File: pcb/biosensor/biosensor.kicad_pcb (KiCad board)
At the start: 2 copper layers, 75 x 65.5 mm, 34 parts, among them J1 Screw_Terminal_01x03, J2 Conn_01x02_Female, P1 USB_C_Plug_USB2.0, SW1 SW_DIP_x01, U1 DW01, U2 TP4056, U3 FS8205A, U4 LM2621

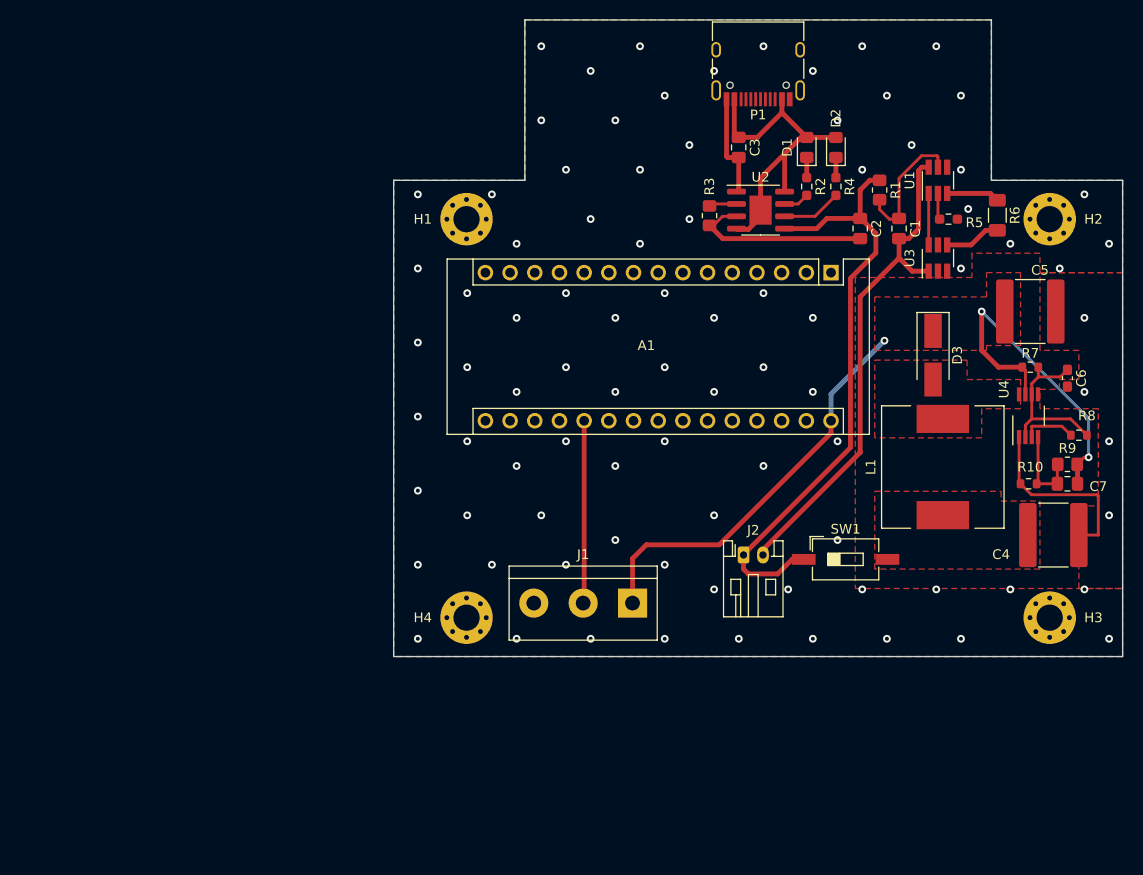
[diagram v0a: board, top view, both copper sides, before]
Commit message: final update?
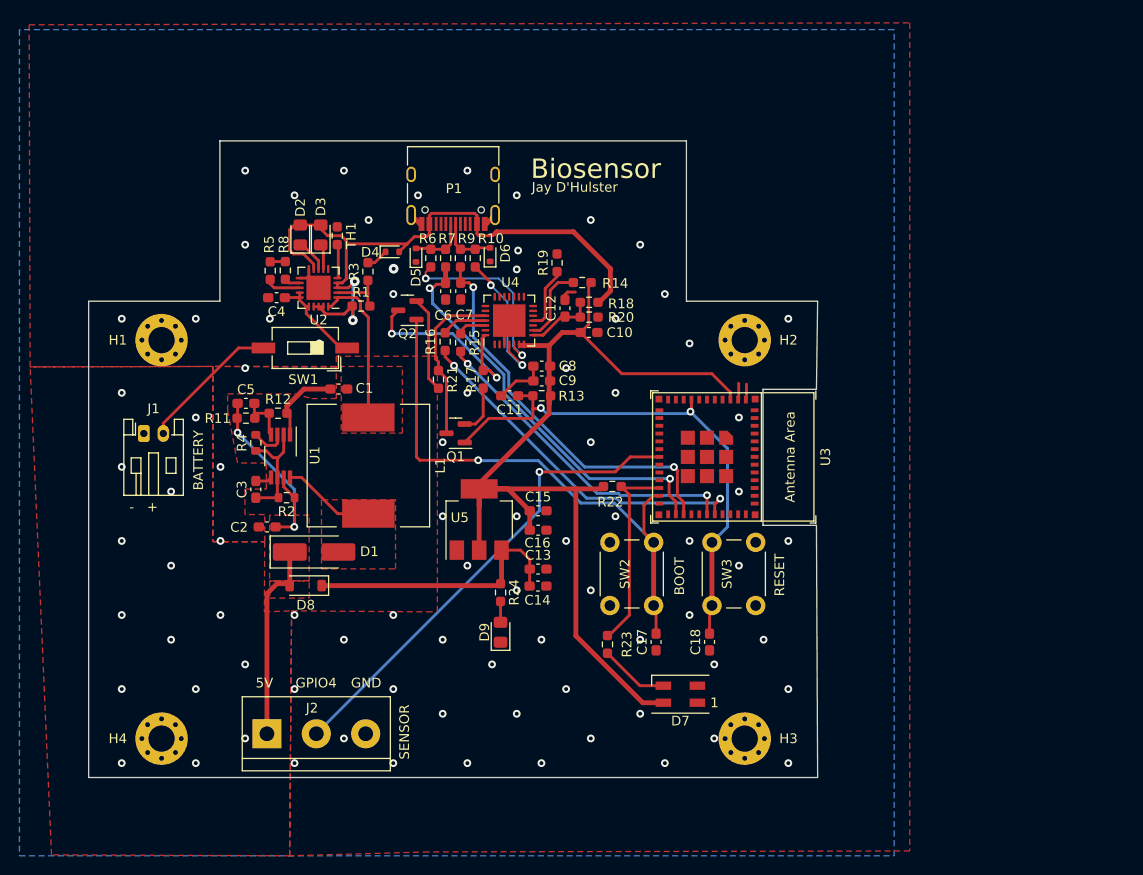
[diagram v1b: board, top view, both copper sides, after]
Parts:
- removed A1: Arduino_Nano_v3.x, Module:Arduino_Nano
- added C10: 10µF/25V/(20%), Capacitor_SMD:C_0603_1608Metric_Pad1.08x0.95mm_HandSolder, F.Cu at (153.6, 86.2)
- added C11: 1µF/16V(10%), Capacitor_SMD:C_0603_1608Metric_Pad1.08x0.95mm_HandSolder, F.Cu at (145.4, 92.7)
- added C12: 1µF/16V(10%), Capacitor_SMD:C_0603_1608Metric_Pad1.08x0.95mm_HandSolder, F.Cu at (151.1, 83.7)
- added C13: 10µF/25V(20%), Capacitor_SMD:C_0603_1608Metric_Pad1.08x0.95mm_HandSolder, F.Cu at (148.4, 110.5)
- added C14: 0.1µF/50V(10%), Capacitor_SMD:C_0603_1608Metric_Pad1.08x0.95mm_HandSolder, F.Cu at (148.3, 112.2)
- added C15: 0.1µF/50V(10%), Capacitor_SMD:C_0603_1608Metric_Pad1.08x0.95mm_HandSolder, F.Cu at (148.4, 104.5)
- added C16: 10µF/25V(20%), Capacitor_SMD:C_0603_1608Metric_Pad1.08x0.95mm_HandSolder, F.Cu at (148.4, 106.5)
- added C17: 0.1µF/50V(10%)(NC), Capacitor_SMD:C_0603_1608Metric_Pad1.08x0.95mm_HandSolder, F.Cu at (160.5, 118.0)
- added C18: 0.1µF/50V(10%)(NC), Capacitor_SMD:C_0603_1608Metric_Pad1.08x0.95mm_HandSolder, F.Cu at (166.0, 118.0)
- added C8: 10µF/25V(20%), Capacitor_SMD:C_0603_1608Metric_Pad1.08x0.95mm_HandSolder, F.Cu at (148.7, 89.6)
- added C9: 0.1µF/50V(10%), Capacitor_SMD:C_0603_1608Metric_Pad1.08x0.95mm_HandSolder, F.Cu at (148.7, 91.1)
- added D4: LESD5D.0CT1G, Diode_SMD:D_SOD-523, F.Cu at (133.4, 77.9)
- added D5: LESD5D.0CT1G, Diode_SMD:D_SOD-523, F.Cu at (135.8, 78.2)
- added D6: LESD5D.0CT1G, Diode_SMD:D_SOD-523, F.Cu at (143.4, 78.2)
- added D7: SK6812MINI, LED_SMD:LED_SK6812MINI_PLCC4_3.5x3.5mm_P1.75mm, F.Cu at (163.0, 123.4)
- added D8: 1N5819HW-7-F, Diode_SMD:D_SOD-123, F.Cu at (124.5, 112.2)
- added D9: RED, LED_SMD:LED_0805_2012Metric_Pad1.15x1.40mm_HandSolder, F.Cu at (144.5, 117.0)
- added Q1: L8050QLT1G, Package_TO_SOT_SMD:SOT-23, F.Cu at (139.9, 96.5)
- added Q2: L8050QLT1G, Package_TO_SOT_SMD:SOT-23, F.Cu at (134.9, 83.9)
- added R11: 150K, Resistor_SMD:R_0603_1608Metric_Pad0.98x0.95mm_HandSolder, F.Cu at (118.3, 95.0)
- added R12: 50K, Resistor_SMD:R_0603_1608Metric_Pad0.98x0.95mm_HandSolder, F.Cu at (121.6, 94.5)
- added R13: 10K(1%), Resistor_SMD:R_0603_1608Metric_Pad0.98x0.95mm_HandSolder, F.Cu at (148.7, 92.7)
- added R14: 1K(1%), Resistor_SMD:R_0603_1608Metric_Pad0.98x0.95mm_HandSolder, F.Cu at (152.9, 81.0)
- added R15: 0(1%), Resistor_SMD:R_0603_1608Metric_Pad0.98x0.95mm_HandSolder, F.Cu at (140.4, 87.2)
- added R16: 0(1%), Resistor_SMD:R_0603_1608Metric_Pad0.98x0.95mm_HandSolder, F.Cu at (138.8, 87.1)
- added R17: 10K(1%), Resistor_SMD:R_0603_1608Metric_Pad0.98x0.95mm_HandSolder, F.Cu at (142.7, 91.0)
- added R18: 22.1K(1%), Resistor_SMD:R_0603_1608Metric_Pad0.98x0.95mm_HandSolder, F.Cu at (153.6, 83.1)
- added R19: 10K(1%)(NC), Resistor_SMD:R_0603_1608Metric_Pad0.98x0.95mm_HandSolder, F.Cu at (150.3, 79.0)
- added R20: 47.5K(1%), Resistor_SMD:R_0603_1608Metric_Pad0.98x0.95mm_HandSolder, F.Cu at (153.6, 84.6)
- added R21: 10K(1%), Resistor_SMD:R_0603_1608Metric_Pad0.98x0.95mm_HandSolder, F.Cu at (138.1, 91.0)
- added R22: 10K(1%), Resistor_SMD:R_0603_1608Metric_Pad0.98x0.95mm_HandSolder, F.Cu at (156.0, 102.0)
- added R23: 0(1%), Resistor_SMD:R_0603_1608Metric_Pad0.98x0.95mm_HandSolder, F.Cu at (155.5, 118.2)
- added R24: 5.1K(1%), Resistor_SMD:R_0603_1608Metric_Pad0.98x0.95mm_HandSolder, F.Cu at (144.5, 112.9)
- added SW2: SW_Push, Button_Switch_THT:SW_PUSH_6mm, F.Cu at (160.2, 107.8)
- added SW3: SW_Push, Button_Switch_THT:SW_PUSH_6mm, F.Cu at (166.2, 114.2)
- added TH1: 16K, Resistor_SMD:R_0603_1608Metric_Pad0.98x0.95mm_HandSolder, F.Cu at (127.7, 76.2)
- added U5: SGM2212-3.3XKC3G/TR, Package_TO_SOT_SMD:SOT-223-3_TabPin2, F.Cu at (142.3, 105.4)
- C1: value 0.1uF -> 22uF; footprint Capacitor_SMD:C_0805_2012Metric_Pad1.18x1.45mm_HandSolder -> Capacitor_SMD:C_0603_1608Metric_Pad1.08x0.95mm_HandSolder
- C2: value 10uF -> 68uF; footprint Capacitor_SMD:C_0805_2012Metric_Pad1.18x1.45mm_HandSolder -> Capacitor_SMD:C_0603_1608Metric_Pad1.08x0.95mm_HandSolder
- C3: value 0.1uF -> 100nF; footprint Capacitor_SMD:C_0805_2012Metric_Pad1.18x1.45mm_HandSolder -> Capacitor_SMD:C_0603_1608Metric_Pad1.08x0.95mm_HandSolder
- C4: value 22uF -> 10µF; footprint Capacitor_SMD:C_2225_5664Metric_Pad1.80x6.60mm_HandSolder -> Capacitor_SMD:C_0603_1608Metric_Pad1.08x0.95mm_HandSolder
- C5: value 68uF -> 39pF; footprint Capacitor_SMD:C_2225_5664Metric_Pad1.80x6.60mm_HandSolder -> Capacitor_SMD:C_0603_1608Metric_Pad1.08x0.95mm_HandSolder
- C6: value 100nF -> 22pF/50V/(5%)(NC)
- C7: value 39pF -> 22pF/50V/(5%)(NC); footprint Capacitor_SMD:C_0805_2012Metric_Pad1.18x1.45mm_HandSolder -> Capacitor_SMD:C_0603_1608Metric_Pad1.08x0.95mm_HandSolder
- D1: value RED -> SS34; footprint LED_SMD:LED_0805_2012Metric_Pad1.15x1.40mm_HandSolder -> Diode_SMD:D_SMA_Handsoldering
- D2: value GREEN -> Opladen
- D3: value SS34 -> Klaar; footprint Diode_SMD:D_SMA_Handsoldering -> LED_SMD:LED_0805_2012Metric_Pad1.15x1.40mm_HandSolder
- J1: value Screw_Terminal_01x03 -> Conn_01x02_Female; footprint TerminalBlock:TerminalBlock_bornier-3_P5.08mm -> Connector_JST:JST_PH_S2B-PH-K_1x02_P2.00mm_Horizontal
- J2: value Conn_01x02_Female -> Screw_Terminal_01x03; footprint Connector_JST:JST_PH_S2B-PH-K_1x02_P2.00mm_Horizontal -> TerminalBlock:TerminalBlock_bornier-3_P5.08mm
- R1: value 100 -> 270K; footprint Resistor_SMD:R_0805_2012Metric_Pad1.20x1.40mm_HandSolder -> Resistor_SMD:R_0603_1608Metric_Pad0.98x0.95mm_HandSolder
- R10: value 50K -> 0(1%); footprint Resistor_SMD:R_0603_1608Metric -> Resistor_SMD:R_0603_1608Metric_Pad0.98x0.95mm_HandSolder
- R2: value 1k -> 500R; footprint Resistor_SMD:R_0603_1608Metric_Pad0.98x0.95mm_HandSolder -> Resistor_SMD:R_0603_1608Metric
- R3: value 10k -> 100K; footprint Resistor_SMD:R_0805_2012Metric_Pad1.20x1.40mm_HandSolder -> Resistor_SMD:R_0603_1608Metric_Pad0.98x0.95mm_HandSolder
- R4: value 1k -> 200K; footprint Resistor_SMD:R_0603_1608Metric_Pad0.98x0.95mm_HandSolder -> Resistor_SMD:R_0603_1608Metric
- R5: value 1k -> 1K
- R6: value 0R -> 0(1%); footprint Resistor_SMD:R_1206_3216Metric_Pad1.30x1.75mm_HandSolder -> Resistor_SMD:R_0603_1608Metric_Pad0.98x0.95mm_HandSolder
- R7: value 500R -> 0(1%)(NC); footprint Resistor_SMD:R_0603_1608Metric -> Resistor_SMD:R_0603_1608Metric_Pad0.98x0.95mm_HandSolder
- R8: value 200K -> 100K; footprint Resistor_SMD:R_0603_1608Metric -> Resistor_SMD:R_0603_1608Metric_Pad0.98x0.95mm_HandSolder
- R9: value 150K -> 0(1%)(NC); footprint Resistor_SMD:R_0805_2012Metric_Pad1.20x1.40mm_HandSolder -> Resistor_SMD:R_0603_1608Metric_Pad0.98x0.95mm_HandSolder
- U1: value DW01 -> LM2621; footprint Package_TO_SOT_SMD:SOT-23-6_Handsoldering -> Package_SO:VSSOP-8_3.0x3.0mm_P0.65mm
- U2: value TP4056 -> MCP73871; footprint Package_SO:SOIC-8-1EP_3.9x4.9mm_P1.27mm_EP2.29x3mm -> Package_DFN_QFN:QFN-20-1EP_4x4mm_P0.5mm_EP2.5x2.5mm
- U3: value FS8205A -> ESP32-C3-MINI-1; footprint Package_TO_SOT_SMD:SOT-23-6_Handsoldering -> Espressif:ESP32-C3-MINI-1
- U4: value LM2621 -> CP2102N-Axx-xQFN28; footprint Package_SO:VSSOP-8_3.0x3.0mm_P0.65mm -> Package_DFN_QFN:QFN-28-1EP_5x5mm_P0.5mm_EP3.35x3.35mm
- moved C4 83.6 mm to (121.5, 82.6), turned to 180 degrees
- moved R8 83.4 mm to (122.4, 79.8), turned to 90 degrees
- moved C5 81.2 mm to (118.3, 93.5)
- moved U1 73.3 mm to (121.9, 98.9), turned to -90 degrees
- moved R5 70.0 mm to (120.8, 79.8), turned to 90 degrees
- moved C2 68.3 mm to (120.5, 106.2), turned to 180 degrees
- moved R9 66.0 mm to (140.4, 78.5), turned to -90 degrees
- moved D1 65.6 mm to (125.3, 108.7), turned to 0 degrees
- moved C7 65.5 mm to (140.4, 81.9), turned to -90 degrees
- moved R4 65.2 mm to (119.3, 97.5), turned to 90 degrees
- moved C6 64.6 mm to (138.8, 81.9)
- moved D3 64.2 mm to (126.0, 76.1), turned to 90 degrees
- moved R2 62.4 mm to (122.5, 103.2), turned to 180 degrees
- moved R10 61.5 mm to (141.9, 78.5), turned to -90 degrees
- moved R7 61.2 mm to (138.8, 78.5), turned to -90 degrees
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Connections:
- C1 pad 1: Net-(C1-Pad1) -> /Load
- C1 pad 2: BAT- -> GND
- C2 pad 1: BAT+ -> +5V
- C3 pad 1: VIN -> Net-(U1-EN)
- C4 pad 1: OUTVCC -> Net-(U2-V_{BAT_SENSE})
- C5 pad 1: /Vout -> +5V
- C5 pad 2: GND -> Net-(U1-FB)
- C6 pad 1: Net-(C6-Pad1) -> /GPIO18
- C7 pad 1: /Vout -> /GPIO19
- C7 pad 2: Net-(C7-Pad2) -> GND
- D1 pad 1: Net-(D1-Pad1) -> +5V
- D1 pad 2: VIN -> /L1
- D2 pad 1: Net-(D2-Pad1) -> Net-(D2-K)
- D2 pad 2: VIN -> VBUS
- D3 pad 1: /Vout -> Net-(D3-K)
- D3 pad 2: /L1 -> VBUS
- J1 pad 1: /Vout -> GND
- J1 pad 2: Net-(A1-Pad20) -> Net-(J1-Pin_2)
- J2 pad 1: BAT+ -> +5V
- J2 pad 2: BAT- -> /GPIO4
- L1 pad 1: OUTVCC -> /Load
- P1 pad A4: VIN -> VBUS
- P1 pad A6: unconnected-(P1-PadA6) -> Net-(D6-A2)
- P1 pad A7: unconnected-(P1-PadA7) -> Net-(D5-A2)
- P1 pad A9: VIN -> VBUS
- P1 pad B4: VIN -> VBUS
- P1 pad B9: VIN -> VBUS
- R1 pad 1: BAT+ -> VBUS
- R1 pad 2: Net-(C1-Pad1) -> Net-(U2-VPCC)
- R10 pad 1: Net-(C7-Pad2) -> Net-(D6-A2)
- R10 pad 2: GND -> /USB_DP
- R2 pad 1: Net-(D1-Pad1) -> +5V
- R2 pad 2: Net-(R2-Pad2) -> Net-(U1-EN)
- R3 pad 1: Net-(R3-Pad1) -> Net-(U2-VPCC)
- R4 pad 1: Net-(D2-Pad1) -> Net-(U1-EN)
- R4 pad 2: Net-(R4-Pad2) -> Net-(U1-FREQ)
- R5 pad 1: GND -> Net-(U2-PROG1)
- R5 pad 2: Net-(R5-Pad2) -> GND
- R6 pad 1: /OC -> Net-(D5-A2)
- R6 pad 2: /G2 -> /USB_DN
- R7 pad 1: /Vout -> Net-(D5-A2)
- R7 pad 2: Net-(C6-Pad1) -> /GPIO18
- R8 pad 1: Net-(C6-Pad1) -> Net-(U2-PROG3)
- R8 pad 2: Net-(R8-Pad2) -> GND
- R9 pad 1: Net-(C7-Pad2) -> Net-(D6-A2)
- R9 pad 2: /Vout -> /GPIO19
- SW1 pad 1: BAT+ -> Net-(U2-V_{BAT_SENSE})
- SW1 pad 2: OUTVCC -> Net-(J1-Pin_2)
- U1 pad 1: /G1 -> GND
- U1 pad 2: Net-(R5-Pad2) -> Net-(U1-EN)
- U1 pad 3: /OC -> Net-(U1-FREQ)
- U1 pad 4: unconnected-(U1-Pad4) -> Net-(U1-FB)
- U1 pad 5: Net-(C1-Pad1) -> GND
- U1 pad 6: BAT- -> Net-(U1-EN)
- U2 pad 1: GND -> /Load
- U2 pad 2: Net-(R3-Pad1) -> Net-(U2-VPCC)
- U2 pad 3: GND -> VBUS
- U2 pad 4: VIN -> VBUS
- U2 pad 5: BAT+ -> Net-(U2-THERM)
- U2 pad 6: Net-(R4-Pad2) -> unconnected-(U2-~{PG}-Pad6)
- U2 pad 7: Net-(R2-Pad2) -> Net-(D3-K)
- U2 pad 8: VIN -> Net-(D2-K)
- U2 pad 9: VIN -> VBUS
- U3 pad 1: BAT- -> GND
- U3 pad 2: unconnected-(U3-Pad2) -> GND
- U3 pad 3: GND -> +3V3
- U3 pad 4: /G2 -> unconnected-(U3-NC-Pad4)
- U3 pad 6: /G1 -> unconnected-(U3-GPIO3/ADC1_CH3-Pad6)
- U4 pad 1: GND -> unconnected-(U4-~{DCD}-Pad1)
- U4 pad 2: Net-(C6-Pad1) -> unconnected-(U4-~{RI}/CLK-Pad2)
- U4 pad 3: Net-(R8-Pad2) -> GND
- U4 pad 4: Net-(C7-Pad2) -> /USB_DP
- U4 pad 5: GND -> /USB_DN
- U4 pad 6: Net-(C6-Pad1) -> +3V3
- U4 pad 7: /Vout -> +3V3
- U4 pad 8: /L1 -> Net-(U4-VBUS)
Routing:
- net +3V3: track 0.00 -> 105.9 mm
- net /Vout: track 76.9 -> 0.00 mm, vias 3 -> 0
- net VBUS: track 0.00 -> 68.7 mm, vias 0 -> 2
- net BAT+: track 62.9 -> 0.00 mm
- net /GPIO9: track 0.00 -> 57.6 mm, vias 0 -> 1
- net /CHIP_PU: track 0.00 -> 54.8 mm, vias 0 -> 2
- net BAT-: track 51.6 -> 0.00 mm
- net /GPIO4: track 0.00 -> 49.5 mm, vias 0 -> 1
- net +5V: track 0.00 -> 42.9 mm, vias 0 -> 2
- net /GPIO18: track 0.00 -> 42.1 mm, vias 0 -> 2
- net /GPIO19: track 0.00 -> 40.9 mm, vias 0 -> 2
- net /U0TXD: track 0.00 -> 37.2 mm, vias 0 -> 2
- net VIN: track 33.9 -> 0.00 mm
- net /U0RXD: track 0.00 -> 33.8 mm, vias 0 -> 2
- net Net-(D8-K): track 0.00 -> 27.6 mm
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- added copper zone on F.Cu, net +5V
- added copper zone on F.Cu, net /Load
- removed copper zone on F.Cu, net /Vout
- removed copper zone on F.Cu, net OUTVCC
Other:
- outline, holes or cut-outs redrawn
- board text added: "- +"
- board text added: "5V"
- board text added: "BATTERY"
- board text added: "BOOT"
- board text added: "Biosensor"
- board text added: "GND"
- board text added: "GPIO4"
- board text added: "Jay D'Hulster"
- board text added: "RESET"
- board text added: "SENSOR"
